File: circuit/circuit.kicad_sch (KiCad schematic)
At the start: 9 parts, among them J1 AC_Input, J2 Device_Output, SW2 SW_DPST, SW3 SW_SPST_Lamp

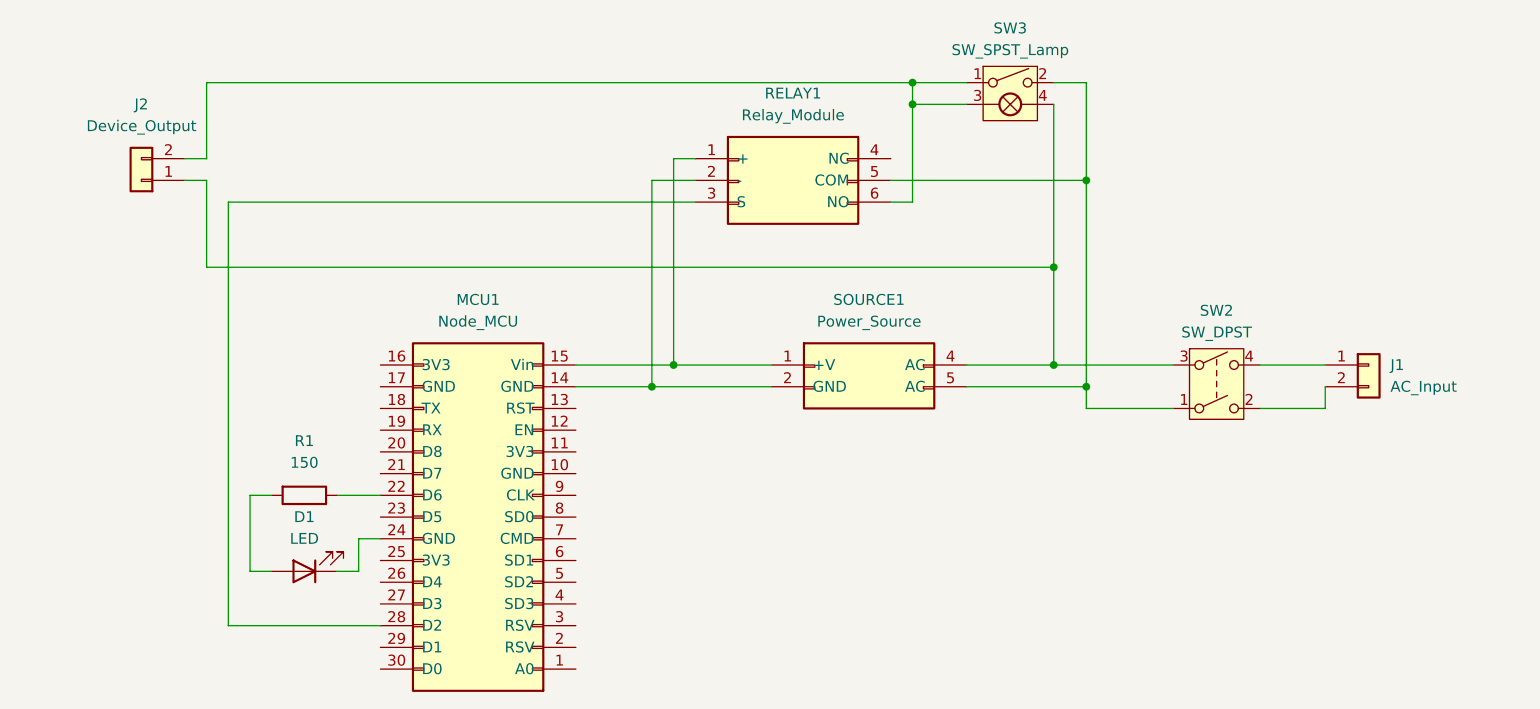
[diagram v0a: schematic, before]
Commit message: Add project screenshots
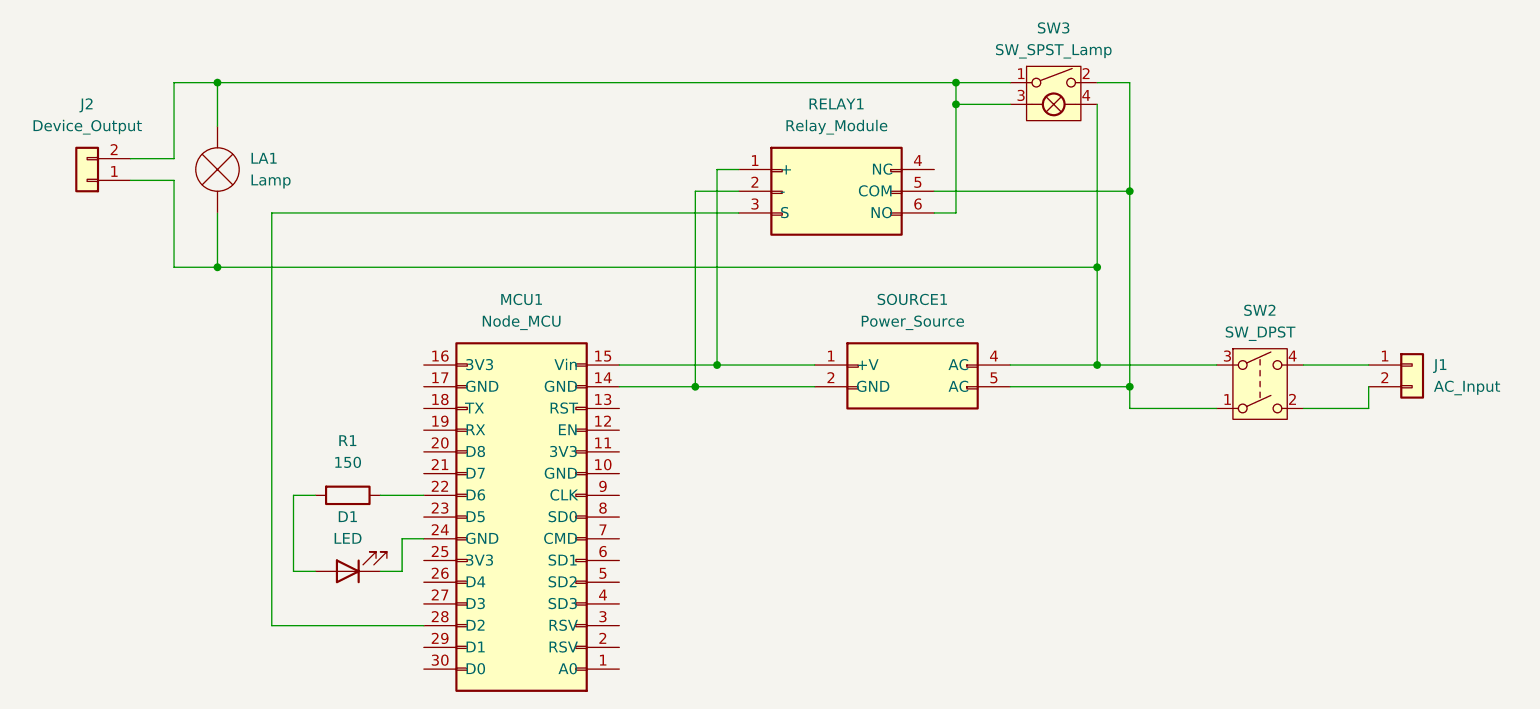
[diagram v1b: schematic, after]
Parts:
- added LA1: Lamp, symbol Device:Lamp
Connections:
- net at J2.2 (Pin_2), RELAY1.6 (NO), SW3.1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: now also LA1.2 (+)
- net at J2.1 (Pin_1), SOURCE1.4 (AC), SW2.3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: now also LA1.1 (-)
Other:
- moved on the sheet: D1, J1, J2, MCU1, R1, RELAY1, SOURCE1, SW2, SW3
